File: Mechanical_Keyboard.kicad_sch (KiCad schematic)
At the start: 125 parts, among them SW1 MX, SW10 MX, SW11 MX, SW12 MX, SW13 MX, SW14 MX, SW15 MX, SW16 MX, SW17 MX, SW18 MX, SW19 MX, SW2 MX, SW20 MX, SW21 MX, SW22 MX, SW23 MX, SW24 MX, SW25 MX, SW26 MX, SW27 MX, SW28 MX, SW29 MX, SW3 MX, SW30 MX, SW31 MX, SW32 MX, SW33 MX, SW34 MX, SW35 MX, SW36 MX, SW37 MX, SW38 MX, SW39 MX, SW4 MX, SW40 MX, SW41 MX, SW42 MX, SW43 MX, SW44 MX, SW46 MX, SW47 MX, SW48 MX, SW49 MX, SW5 MX, SW51 MX, SW52 MX, SW53 MX, SW54 MX, SW56 MX, SW57 MX, SW58 MX, SW59 MX, SW6 MX, SW61 MX, SW62 MX, SW63 MX, SW64 MX, SW66 MX, SW67 MX, SW7 MX, SW8 MX, SW9 MX, U1 ATmega32U4-A

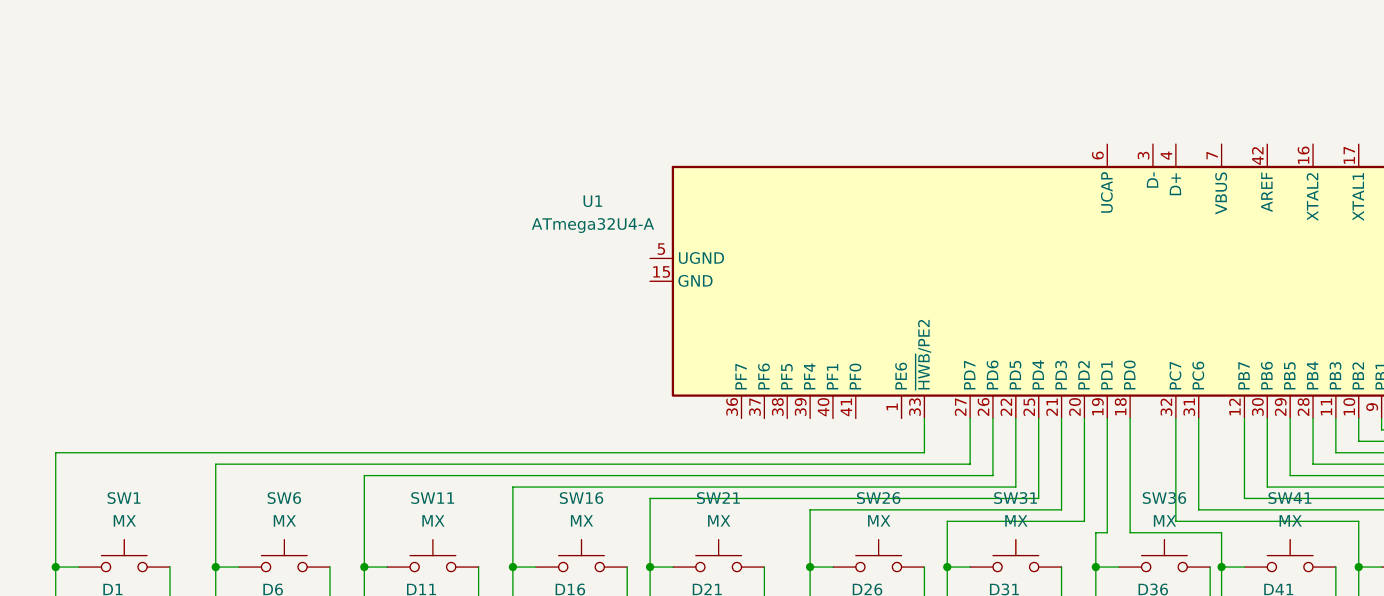
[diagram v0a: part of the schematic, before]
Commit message: Add files via upload
lots of research and a little sketch
https://www.reddit.com/r/PrintedCircuitBoard/comments/kvat9d/usb_type_c_with_atmega32u4/
https://www.digikey.com/en/products/detail/gct/USB4110-GF-A/10384547
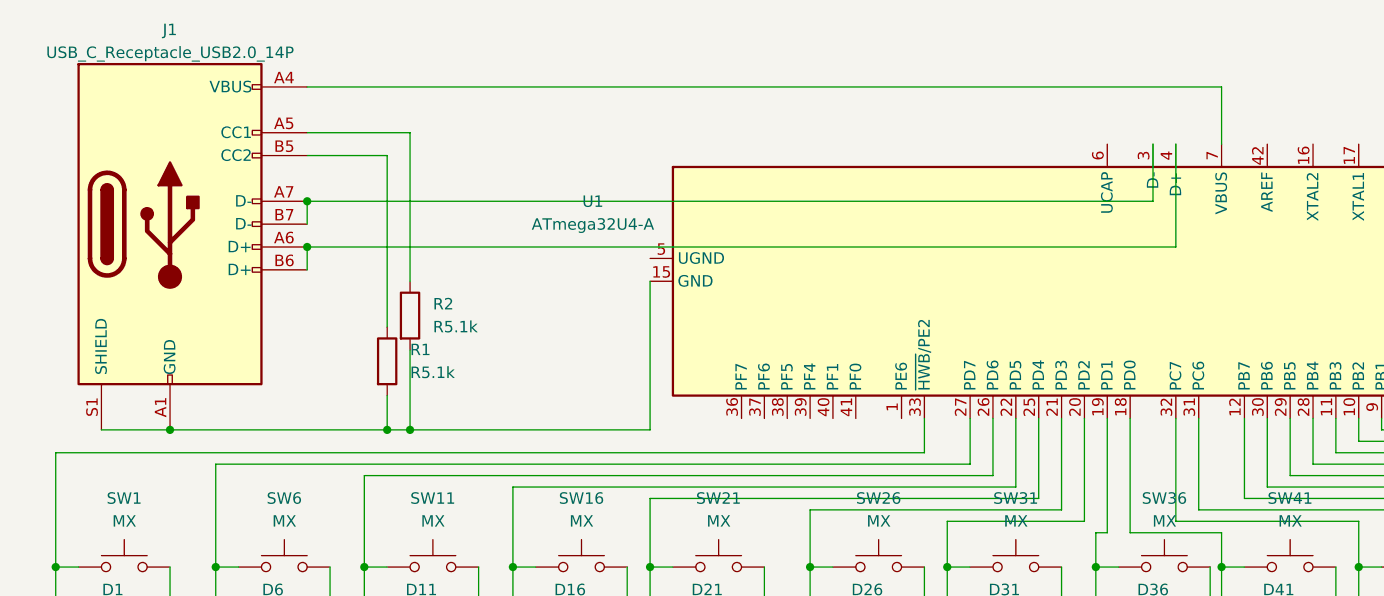
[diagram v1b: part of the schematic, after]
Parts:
- added J1: USB_C_Receptacle_USB2.0_14P, Connector_USB:USB_C_Receptacle_GCT_USB4085, symbol Connector:USB_C_Receptacle_USB2.0_14P
- added R1, R2: R5.1k, Resistor_SMD:R_1206_3216Metric, symbol Device:R
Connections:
- net at U1.15 (GND), U1.23 (GND), U1.35 (GND)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: now also J1.A1 (GND), J1.A12 (GND), J1.B1 (GND), J1.B12 (GND), J1.S1 (SHIELD), R1.2, R2.2
- net at U1.3 (D-): now also J1.A7 (D-), J1.B7 (D-)
- net at U1.4 (D+): now also J1.A6 (D+), J1.B6 (D+)
- net at U1.7 (VBUS): now also J1.A4 (VBUS), J1.A9 (VBUS), J1.B4 (VBUS), J1.B9 (VBUS)
- new net: J1.B5 (CC2), R1.1
- new net: J1.A5 (CC1), R2.1

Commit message: Add files via upload
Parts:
- D1, D10, D11, D12, D13, D14, D15, D16, D17, D18, D19, D2, D20, D21, D22, D23, D24, D25, D26, D27, D28, D29, D3, D30, D31, D32, D33, D34, D35, D36, D37, D38, D39, D4, D40, D41, D42, D43, D44, D46, D47, D48, D49, D5, D51, D52, D53, D54, D56, D57, D58, D59, D6, D61, D62, D63, D64, D66, D67, D7, D8, D9: footprint (none) -> Diode_SMD:D_SOD-123
- SW1, SW11, SW12, SW13, SW14, SW16, SW17, SW18, SW19, SW20, SW21, SW22, SW23, SW24, SW26, SW27, SW28, SW29, SW31, SW32, SW33, SW34, SW36, SW37, SW38, SW39, SW41, SW42, SW43, SW44, SW46, SW47, SW48, SW49, SW51, SW52, SW53, SW54, SW56, SW57, SW58, SW59, SW6, SW61, SW62, SW66, SW7, SW8: footprint (none) -> Button_Switch_Keyboard:SW_Cherry_MX_1.00u_PCB
- SW10, SW15, SW30, SW35, SW4, SW40, SW5: footprint (none) -> Button_Switch_Keyboard:SW_Cherry_MX_1.25u_PCB
- SW2: footprint (none) -> Button_Switch_Keyboard:SW_Cherry_MX_1.50u_PCB
- SW25: footprint (none) -> Button_Switch_Keyboard:SW_Cherry_MX_6.25u_PCB
- SW3, SW67: footprint (none) -> Button_Switch_Keyboard:SW_Cherry_MX_1.75u_PCB
- SW63, SW9: footprint (none) -> Button_Switch_Keyboard:SW_Cherry_MX_2.00u_PCB
- SW64: footprint (none) -> Button_Switch_Keyboard:SW_Cherry_MX_2.25u_PCB
